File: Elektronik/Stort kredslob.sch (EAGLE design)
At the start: 35 parts, among them T1 BC457, T2 BC457, T3 BC457, T5 BC457, T6 BC457, T7 BC457, X2 22-23-2031

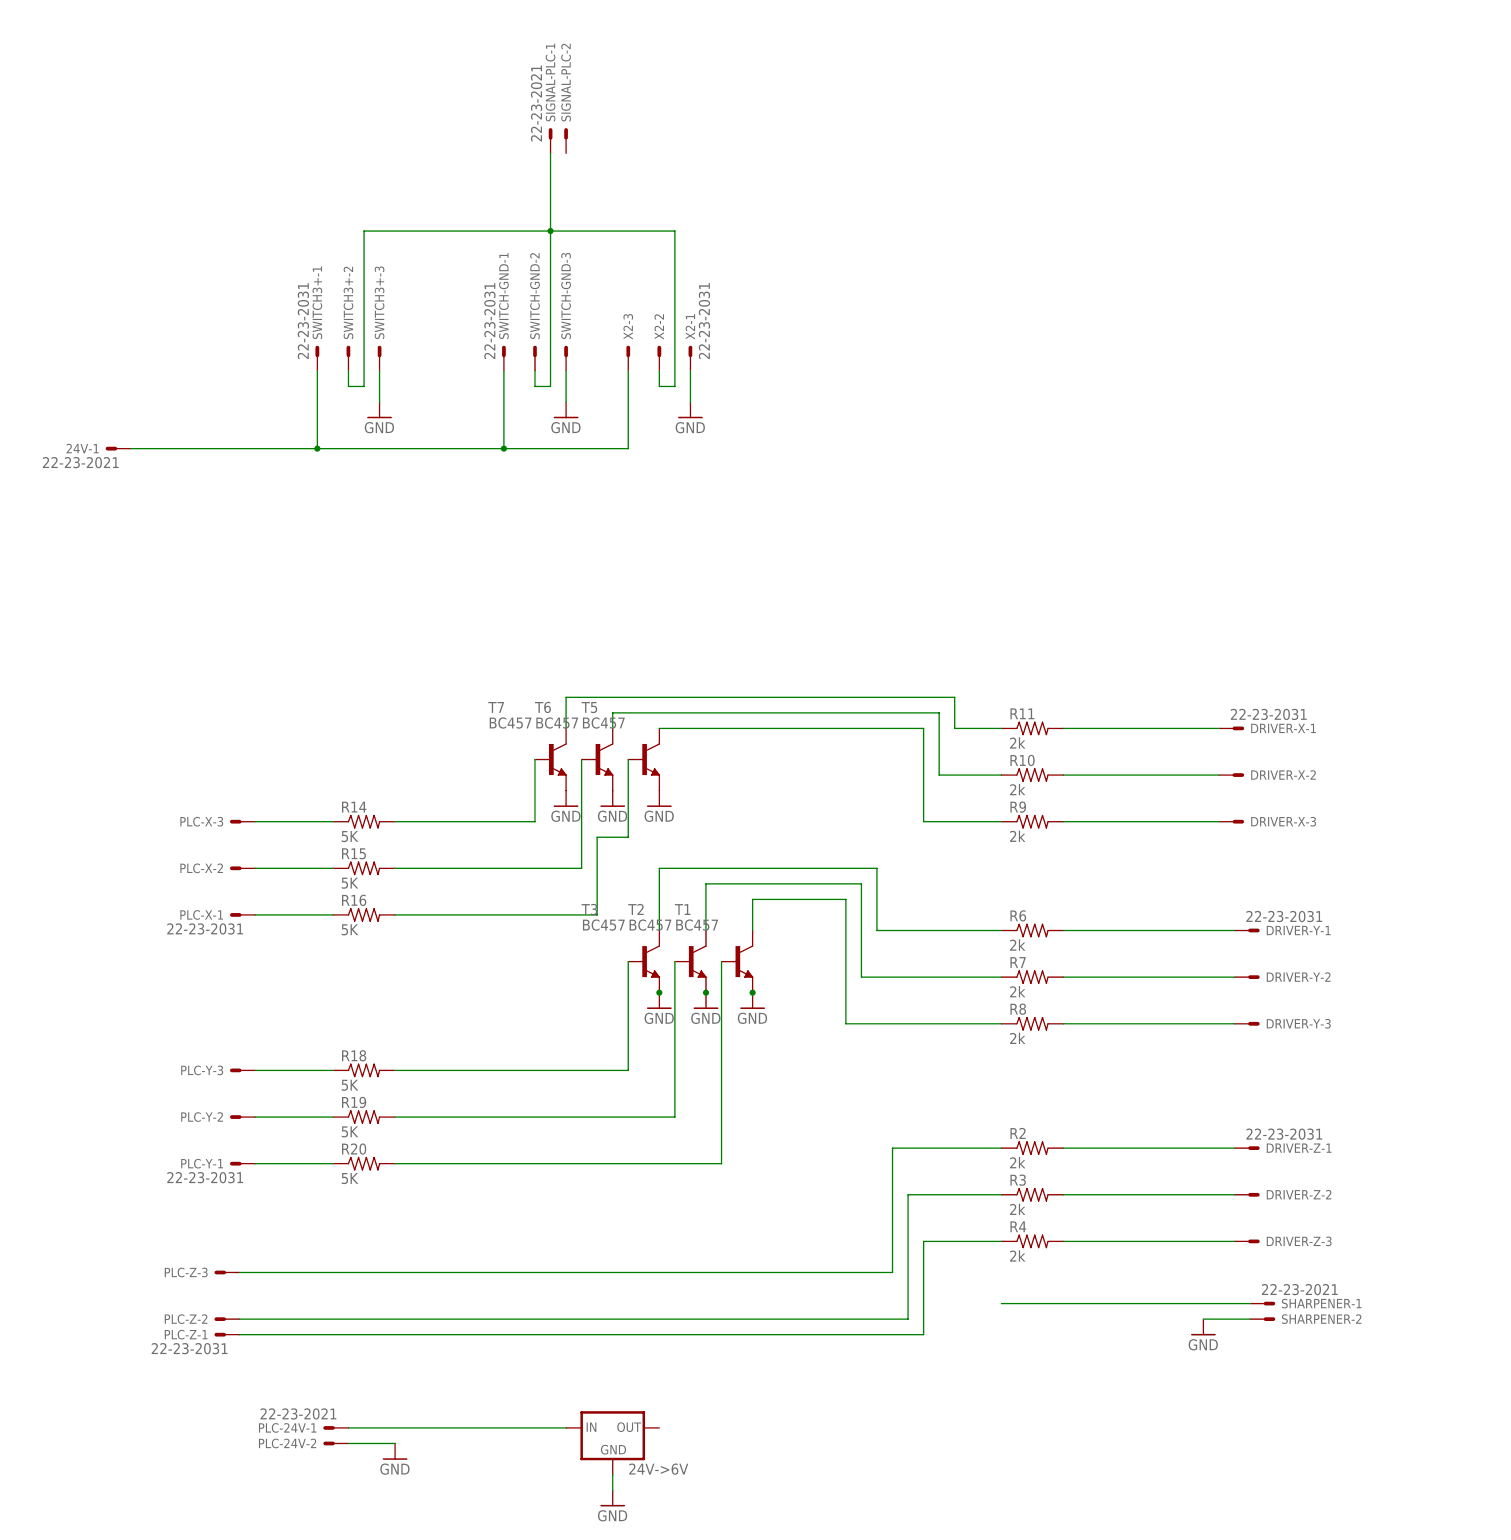
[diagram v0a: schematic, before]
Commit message: PCB-2
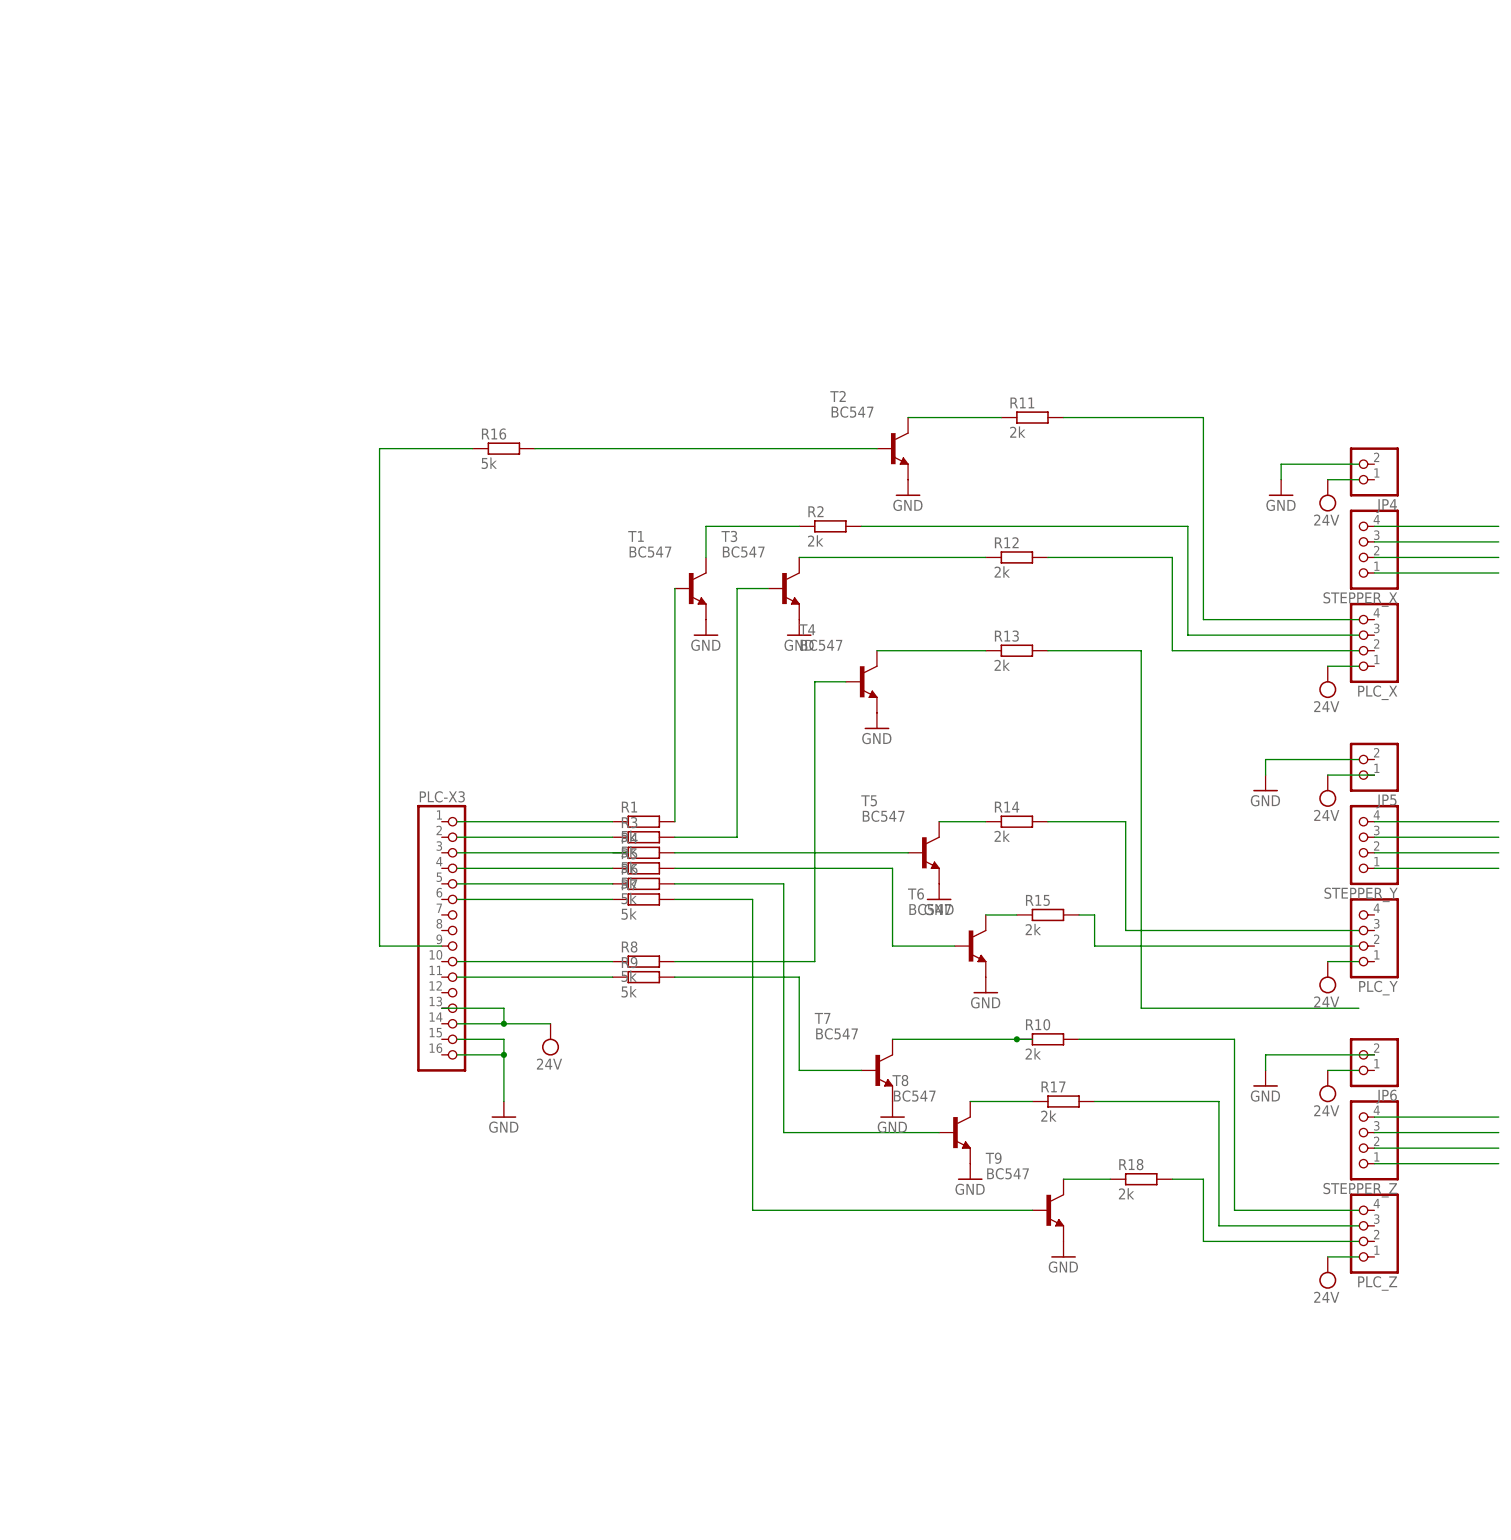
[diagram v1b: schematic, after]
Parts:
- removed 24V, PLC-24V, SHARPENER, SIGNAL-PLC: 22-23-2021, con-molex:22-23-2021
- removed 24V->6V: (no value), v-reg:78XXS
- removed DRIVER-X, DRIVER-Y, DRIVER-Z, PLC-X, PLC-Y, PLC-Z, SWITCH-GND, SWITCH3+, X2: 22-23-2031, con-molex:22-23-2031
- removed R19, R20: 5K, rcl:R-US_0204/7
- added JP4, JP5, JP6: (no value), pinhead:PINHD-1X2
- added PLC-X3: (no value), pinhead:PINHD-1X16
- added PLC_X, PLC_Y, PLC_Z, STEPPER_X, STEPPER_Y, STEPPER_Z: (no value), pinhead:PINHD-1X4
- added R1, R5: 5k, rcl:R-EU_0207/10
- added R12, R13, R17: 2k, rcl:R-EU_0207/10
- added T4, T8, T9: BC547, transistor:-NPN-TO92-E1
- R10, R11, R2: device rcl:R-US_0204/7 -> rcl:R-EU_0207/10
- R14, R15, R18: value 5K -> 2k; device rcl:R-US_0204/7 -> rcl:R-EU_0207/10
- R16: value 5K -> 5k; device rcl:R-US_0204/7 -> rcl:R-EU_0207/10
- R3, R4, R6, R7, R8, R9: value 2k -> 5k; device rcl:R-US_0204/7 -> rcl:R-EU_0207/10
- T1, T2, T3, T5, T6, T7: value BC457 -> BC547; device transistor:2N3565 -> transistor:-NPN-TO92-E1
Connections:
- removed net N$17: PLC-Y-3.S, R18.1
- new net N$14: STEPPER_Z.2
- new net N$30: R4.2, T5.B
- new net N$36: R5.2, T6.B
- new net N$38: R15.2
- new net N$39: R9.1
- new net N$40: R9.2, T7.B
- new net N$41: R10.1, T7.C
- new net N$42: R6.2, T8.B
- new net N$43: R7.2, T9.B
- new net N$44: R10.2
- new net N$45: R17.1, T8.C
- new net N$46: R17.2
- new net N$47: R18.1, T9.C
- new net N$48: R18.2
- new net VCC: JP5.1, PLC-X3.13
- net GND: now also JP6.2, T4.E, T8.E, T9.E; no longer 24V->6V.GND, PLC-24V-2.S, SHARPENER-2.S, SWITCH-GND-3.S, SWITCH3+-3.S, X2-1.S
- net N$1: now also R1.1; no longer SHARPENER-1.S
- net N$10: now also STEPPER_X.4; no longer R18.2, T3.B
- net N$11: now also STEPPER_Y.1; no longer R19.2, T2.B
- net N$12: now also STEPPER_Z.4; no longer R20.2, T1.B
- net N$13: now also STEPPER_Z.3; no longer 24V->6V.IN, PLC-24V-1.S
- net N$15: now also STEPPER_Z.1; no longer PLC-X-1.S, R16.1
- net N$16: now also R3.1; no longer SIGNAL-PLC-1.S, SWITCH-GND-2.S, SWITCH3+-2.S, X2-2.S
- net N$18: now also R5.1; no longer R8.1, T1.C
- net N$19: now also R6.1; no longer DRIVER-Y-3.S, R8.2
- net N$2: now also R1.2, T1.B; no longer DRIVER-Z-1.S, R2.2
- net N$20: no longer T2.C
- net N$21: now also R11.2; no longer DRIVER-Y-2.S, R7.2
- net N$22: now also PLC-X3.9, R16.1; no longer R6.1, T3.C
- net N$23: now also R11.1, T2.C; no longer DRIVER-Y-1.S, R6.2
- net N$24: now also R16.2, T2.B; no longer PLC-Y-2.S, R19.1
- net N$25: now also R2.2; no longer R9.1, T5.C
- net N$26: now also R12.1, T3.C; no longer DRIVER-X-2.S, R10.2
- net N$27: now also R12.2; no longer R10.1, T6.C
- net N$28: now also R8.1; no longer R11.1, T7.C
- net N$29: now also R3.2, T3.B; no longer PLC-Y-1.S, R20.1
- net N$3: now also R2.1, T1.C; no longer DRIVER-Z-2.S, R3.2
- net N$31: now also R8.2, T4.B; no longer DRIVER-X-1.S, R11.2
- net N$32: now also R13.1, T4.C; no longer DRIVER-X-3.S, R9.2
- net N$33: now also R13.2; no longer PLC-Z-1.S, R4.1
- net N$34: now also R14.1, T5.C; no longer PLC-Z-2.S, R3.1
- net N$35: now also R14.2; no longer PLC-Z-3.S, R2.1
- net N$37: now also R15.1, T6.C; no longer PLC-X-3.S, R14.1
- net N$4: now also STEPPER_X.3; no longer DRIVER-Z-3.S, R4.2
- net N$5: now also STEPPER_X.2; no longer 24V-1.S, SWITCH-GND-1.S, SWITCH3+-1.S, X2-3.S
- net N$6: now also STEPPER_X.1; no longer R14.2, T7.B
- net N$7: now also STEPPER_Y.4; no longer R15.2, T6.B
- net N$8: now also STEPPER_Y.3; no longer R16.2, T5.B
- net N$9: now also STEPPER_Y.2; no longer PLC-X-2.S, R15.1
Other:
- moved on the sheet: T1, T2, T3, T5, T6, T7
